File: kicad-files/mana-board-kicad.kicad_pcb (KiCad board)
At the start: 2 copper layers, 200 x 125 mm, 63 parts, among them U1 Pico, U2 74AHCT1G125

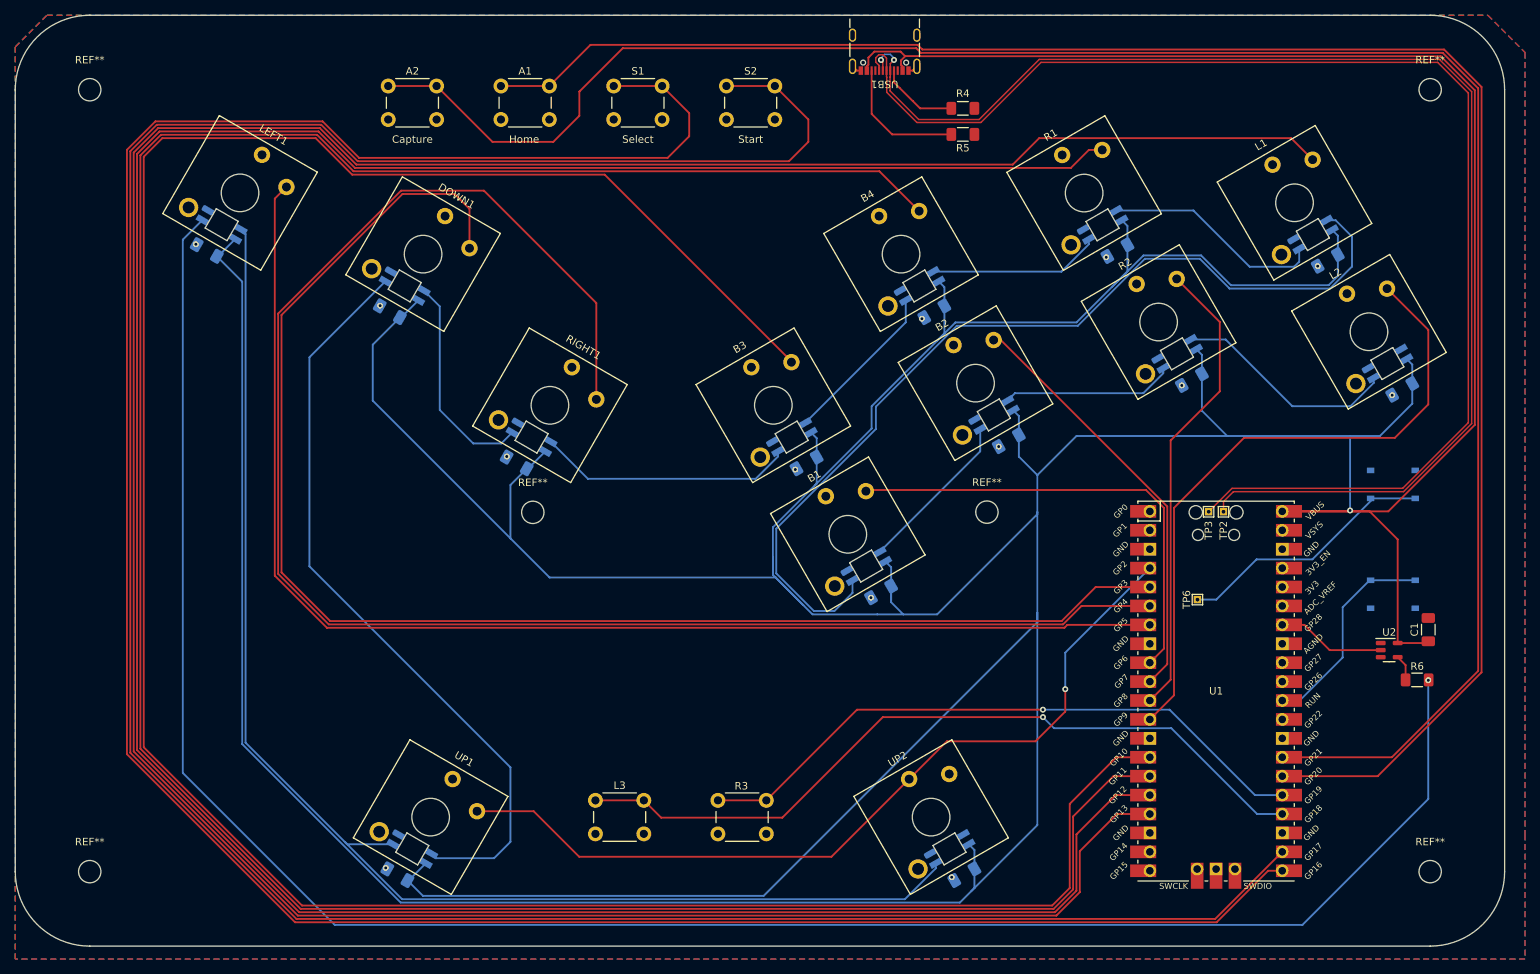
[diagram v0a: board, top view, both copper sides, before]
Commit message: Cleaned up routing, cleanup todo
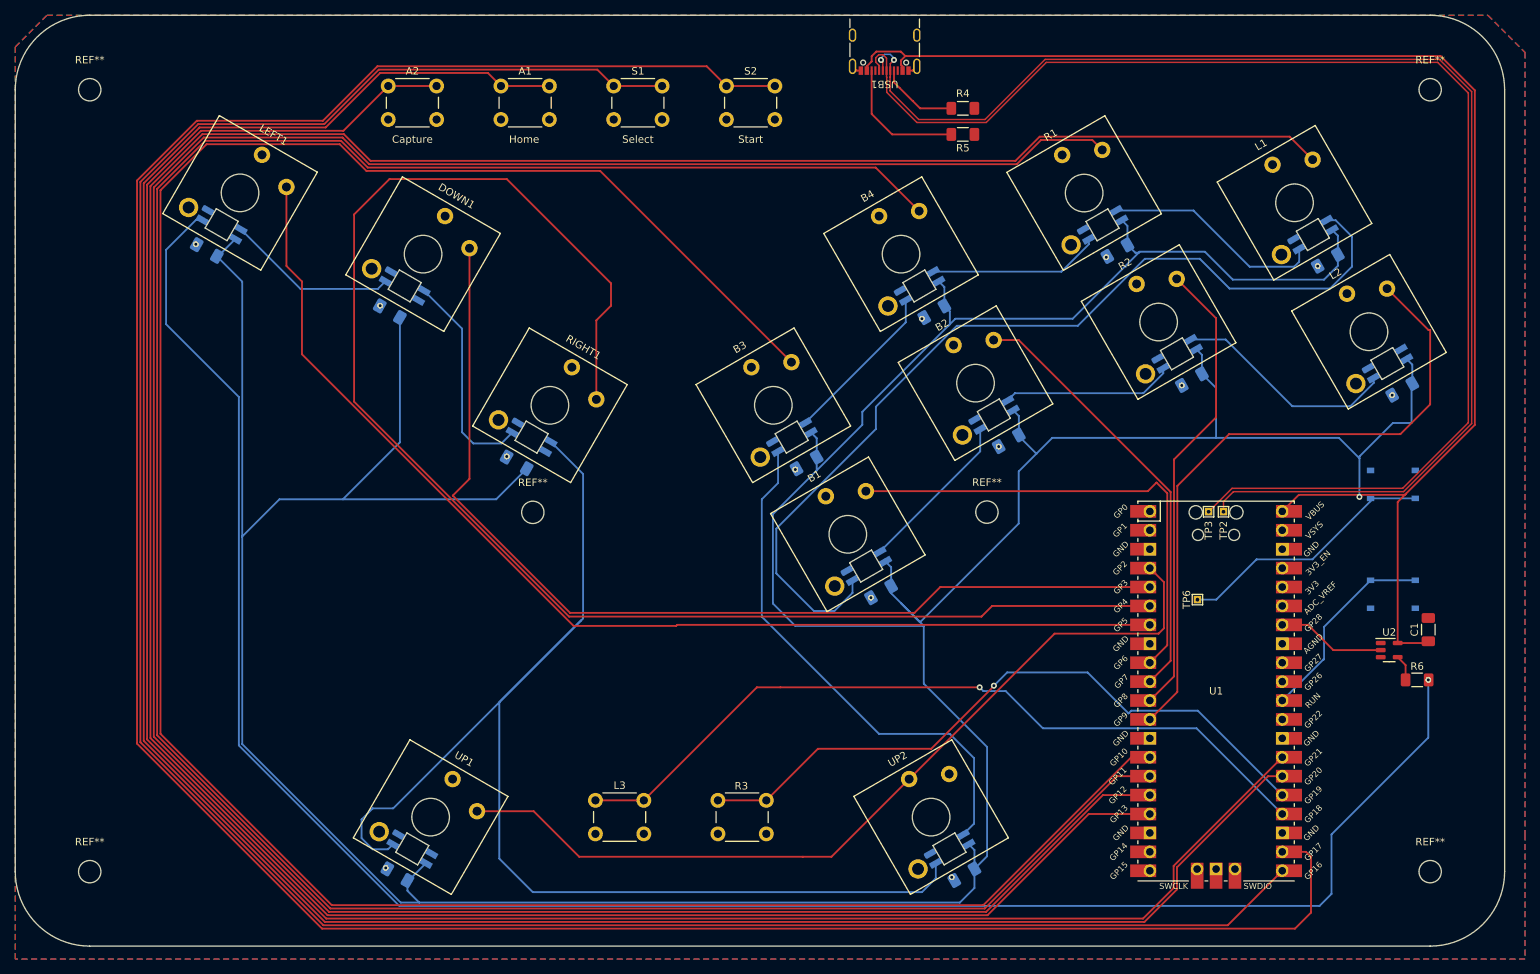
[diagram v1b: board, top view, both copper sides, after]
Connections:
- D13 pad 2: unconnected-(D13-DOUT-Pad2) -> Net-(D13-DOUT)
- D13 pad 4: Net-(D1-DOUT) -> Net-(D13-DIN)
- D2 pad 2: Net-(D2-DOUT) -> unconnected-(D2-DOUT-Pad2)
- D2 pad 4: Net-(D1-DOUT) -> Net-(D13-DIN)
- D3 pad 4: Net-(D2-DOUT) -> Net-(D1-DOUT)
- D4 pad 2: Net-(D4-DOUT) -> Net-(D13-DIN)
- D5 pad 4: Net-(D4-DOUT) -> Net-(D13-DOUT)
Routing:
- net Net-(D13-DIN): track 0.00 -> 173.9 mm
- net 5V: track 931.6 -> 769.0 mm
- net Net-(D1-DOUT): track 179.6 -> 23.2 mm
- net Net-(D2-DOUT): track 102.5 -> 0.00 mm
- net Net-(D13-DOUT): track 0.00 -> 70.3 mm
- net Net-(U1-GPIO20): track 247.5 -> 309.0 mm
- net Net-(U1-GPIO3): track 193.9 -> 135.7 mm
- net Net-(D4-DOUT): track 34.5 -> 0.00 mm
- net Net-(U1-GPIO16): track 343.6 -> 319.0 mm
- net Net-(U1-GPIO21): track 268.2 -> 292.0 mm
- net Net-(U1-GPIO4): track 224.6 -> 203.2 mm
- net Net-(U1-GPIO5): track 173.4 -> 152.4 mm
- net Net-(U1-GPIO10): track 338.6 -> 323.0 mm
- net Net-(U1-GPIO11): track 347.2 -> 332.6 mm
- net Net-(U1-GPIO12): track 369.9 -> 357.3 mm
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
